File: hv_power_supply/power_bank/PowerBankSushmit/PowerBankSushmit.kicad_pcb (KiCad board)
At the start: 2 copper layers, 43 parts, among them J1 NanoFit_RA_TH_02, J2 NanoFit_RA_TH_02, J3 USB-A-S-X-X-SM2, Q1 SSM3K333R, U1 USB_MicroB, U2 MCP73871T-2CCI_ML, U3 TPS61090RSAR

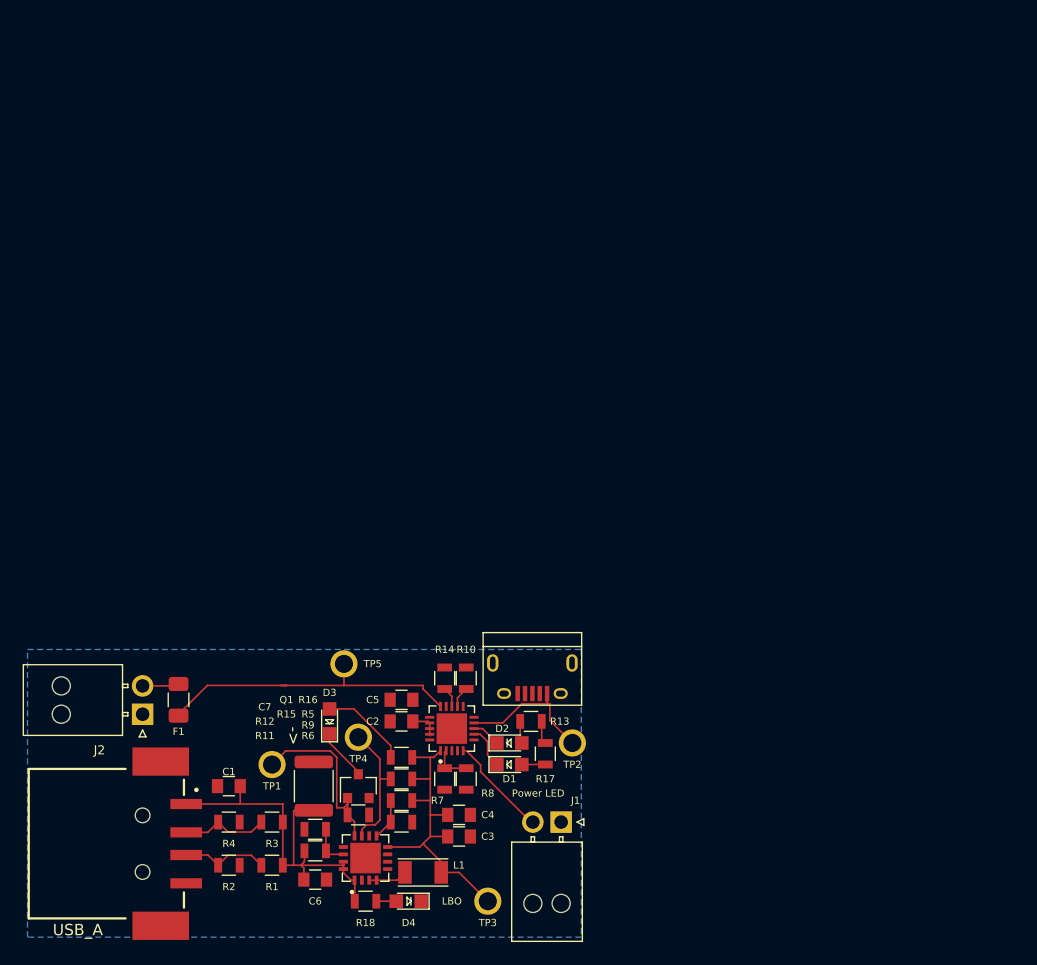
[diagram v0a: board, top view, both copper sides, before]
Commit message: Updated PCB Layout
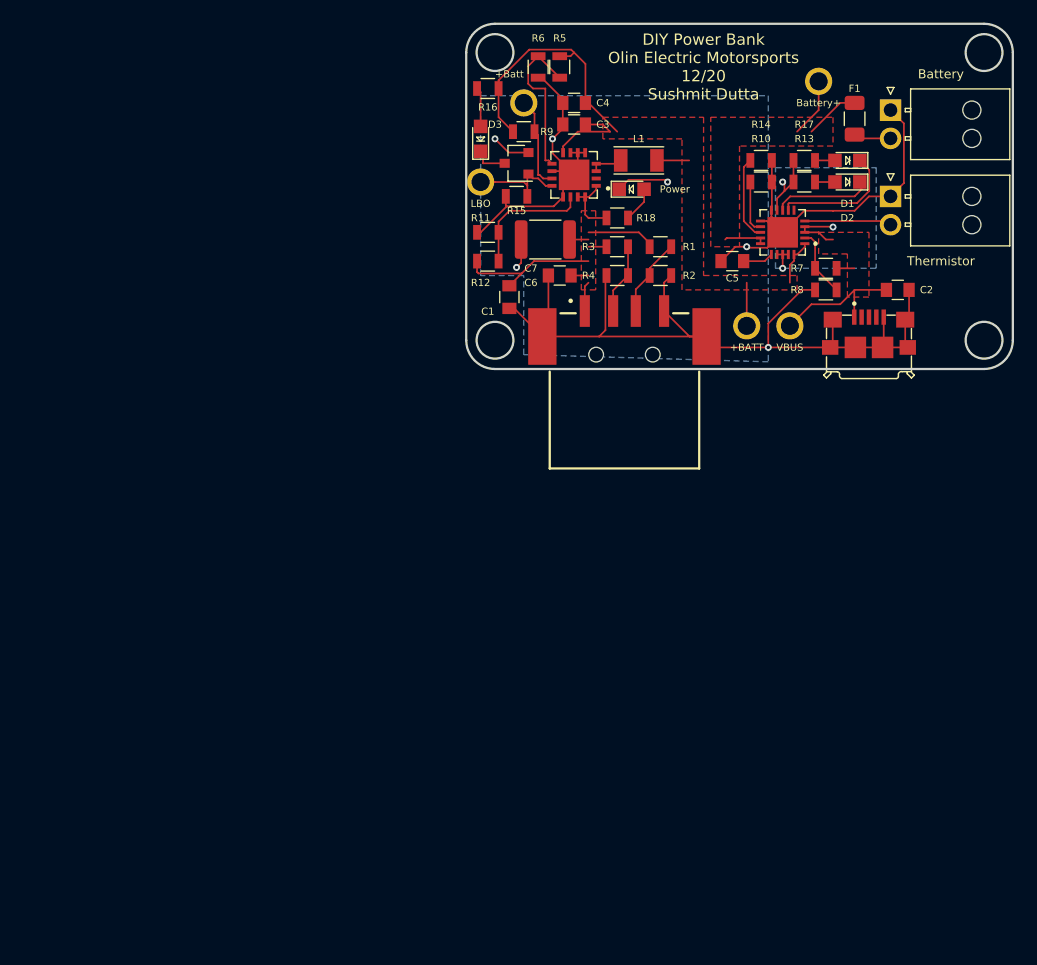
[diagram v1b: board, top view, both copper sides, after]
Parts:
- removed D4: LED_0805, formula:LED_0805_OEM
- removed J1, J2: NanoFit_RA_TH_02, formula:NanoFit_Molex_1x02x2.50mm_Angled_OEM
- removed TP1, TP2, TP3, TP4, TP5: TP, formula:tp_1.6mm
- added +BATT: TP, formula:tp_1.6mm, F.Cu at (236.9, 69.8)
- added +Batt: TP, formula:tp_1.6mm, F.Cu at (217.2, 50.2)
- added Battery: NanoFit_RA_TH_02, formula:NanoFit_Molex_1x02x2.50mm_Angled_OEM, F.Cu at (249.6, 50.8)
- added Battery+: TP, formula:tp_1.6mm, F.Cu at (243.2, 48.3)
- added LBO: TP, formula:tp_1.6mm, F.Cu at (213.1, 57.1)
- added Power : LED_0805, formula:LED_0805_OEM, F.Cu at (226.7, 57.8)
- added Thermistor: NanoFit_RA_TH_02, formula:NanoFit_Molex_1x02x2.50mm_Angled_OEM, F.Cu at (249.6, 58.4)
- added VBUS: TP, formula:tp_1.6mm, F.Cu at (240.7, 69.8)
- U1: value USB_MicroB -> USB-Micro-1981568-1; footprint formula:USB_Micro-B -> formula:TE_1981568-1
- moved F1 78.7 mm to (246.4, 51.6), turned to 90 degrees
- moved R6 67.8 mm to (218.4, 47.0), turned to 270 degrees
- moved R5 66.3 mm to (220.3, 47.0), turned to 270 degrees
- moved L1 65.7 mm to (227.3, 55.2)
- moved R2 64.5 mm to (229.2, 65.4)
- moved R1 64.5 mm to (229.2, 62.9), turned to 0 degrees
- moved R18 64.3 mm to (225.4, 60.3)
- moved C3 63.7 mm to (221.6, 52.1), turned to 180 degrees
- moved C4 63.7 mm to (221.6, 50.2), turned to 180 degrees
- moved U3 63.1 mm to (221.6, 56.5), turned to 180 degrees
- moved D1 61.1 mm to (245.7, 55.2), turned to 180 degrees
- moved J3 60.6 mm to (226.1, 72.4), turned to 0 degrees
- moved R16 59.5 mm to (214.0, 48.9)
- moved R3 59.2 mm to (225.4, 62.9), turned to 0 degrees
- moved R4 59.2 mm to (225.4, 65.4), turned to 180 degrees
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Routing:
- net GND: track 0.17 -> 148.0 mm, vias 0 -> 6
- net /Battery+: track 27.7 -> 13.8 mm
- net +BATT: track 28.8 -> 41.9 mm
- net Net-(R5-Pad2): track 3.66 -> 14.2 mm
- net VBUS: track 17.4 -> 27.6 mm, vias 0 -> 3
- net Net-(R11-Pad2): track 3.57 -> 11.3 mm
- net Net-(D1-Pad1): track 3.84 -> 11.2 mm
- net Net-(Q1-Pad1): track 15.6 -> 8.92 mm
- net Net-(D2-Pad1): track 2.55 -> 8.79 mm
- net Net-(R14-Pad1): track 1.80 -> 7.49 mm
- net Net-(D3-Pad2): track 7.78 -> 3.48 mm
- net Net-(R9-Pad1): track 11.6 -> 8.23 mm
- net Net-(R10-Pad1): track 1.86 -> 4.64 mm
- net Net-(C5-Pad1): track 0.00 -> 2.69 mm
- net Net-(R7-Pad2): track 3.50 -> 6.07 mm
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- added copper zone on F.Cu, net +5V
- added copper zone on F.Cu, net +BATT
- added copper zone on F.Cu, net /Battery+
- added copper zone on B.Cu, net VBUS
- added copper zone on F.Cu, net VBUS
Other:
- board outline added: 48.3 x 30.5 mm
- board text added: "DIY Power Bank Olin Electric Motorsports 12/20 Sushmit Dutta"
- board text removed: "->"
- board text removed: "LBO"
- board text removed: "Power LED"
- board text removed: "USB_A"
